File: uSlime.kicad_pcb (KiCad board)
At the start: 2 copper layers, 22.2 x 29.6 mm, 28 parts, among them J1 USB_C_4-LAYER_PADS, U1 ESP32-C6-WROOM-1-NARROW, U2 AP2112K-3.3TRG1, U3 MCP73831T-2ACI/OT, U5 BNO085, Y1 32.768

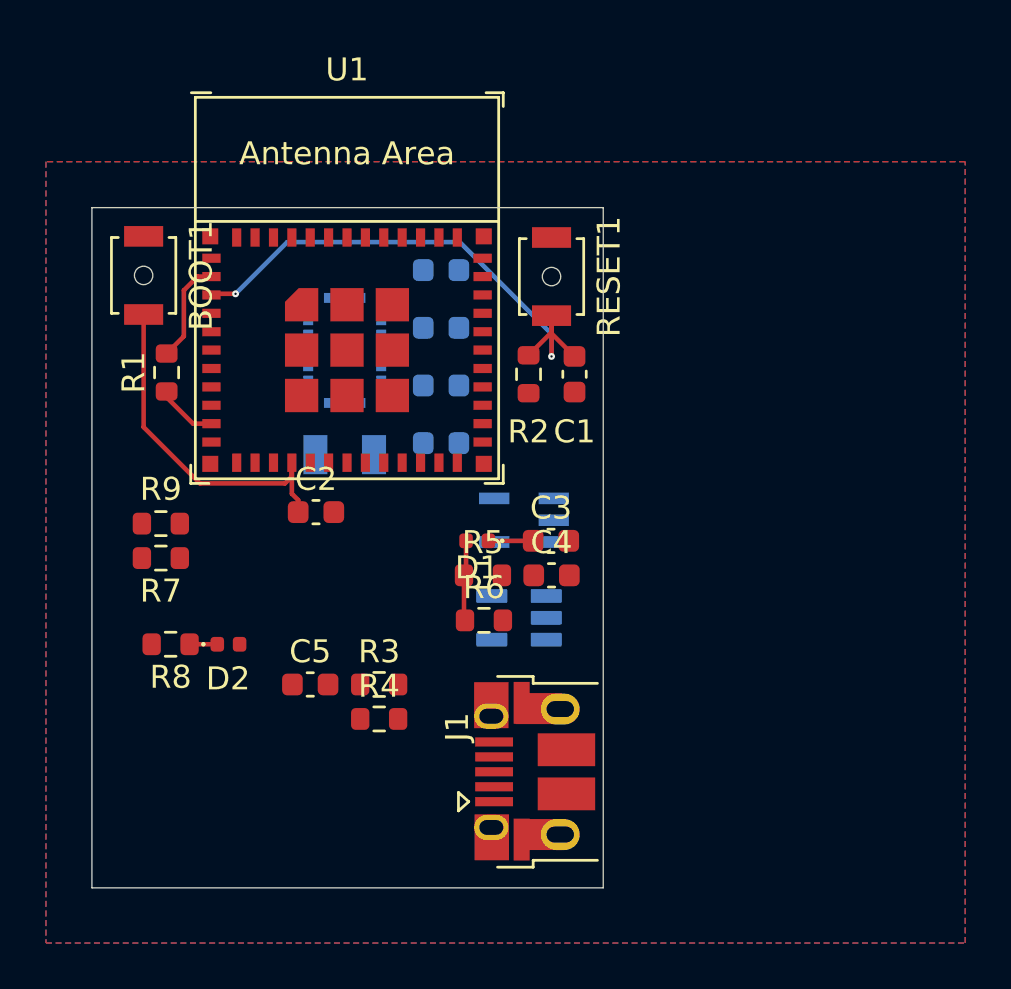
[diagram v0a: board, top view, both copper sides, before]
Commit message: update power
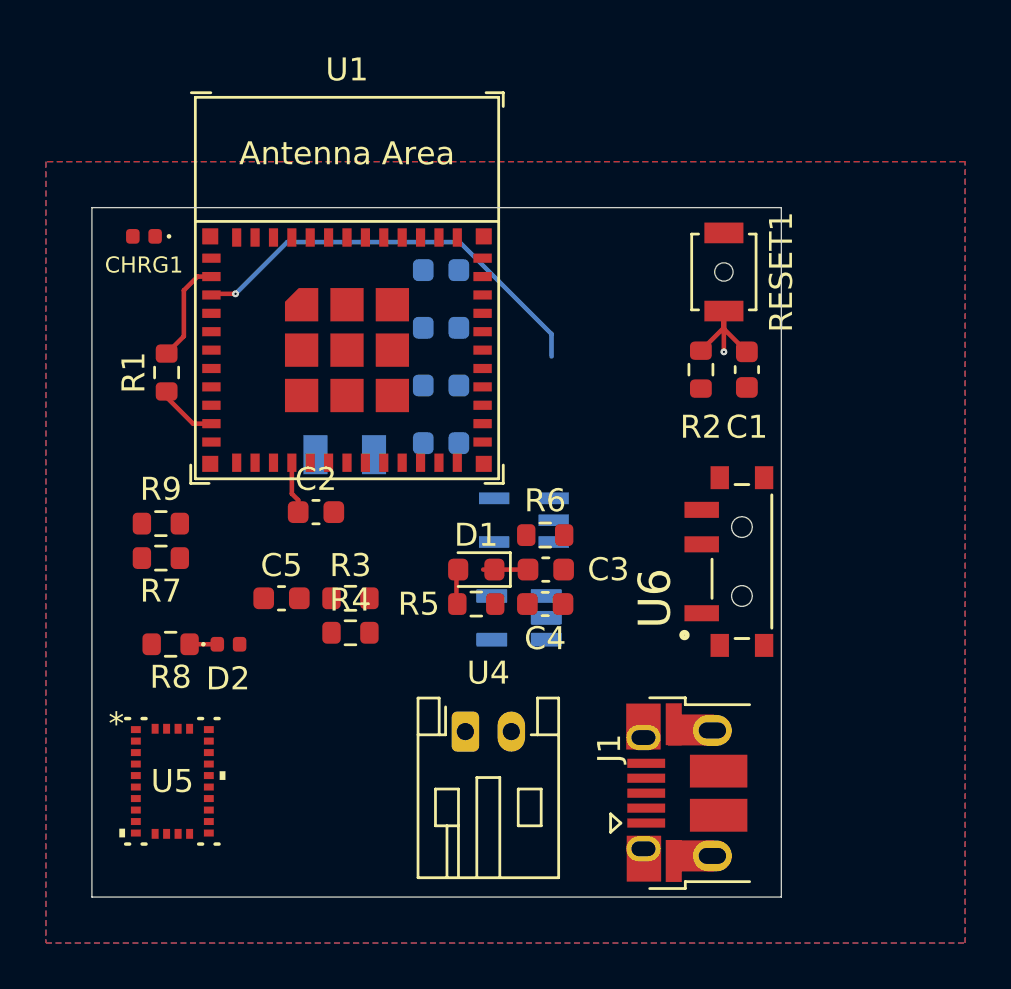
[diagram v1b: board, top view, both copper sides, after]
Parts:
- removed BOOT1: SW_Push, Button_Switch_SMD:SW_SPST_B3U-1000P-B
- added CHRG1: LED, LED_SMD:LED_0402_1005Metric, F.Cu at (102.9, 90.6)
- added U4: S2B-PH-K-S-GW, Connector_JST:JST_PH_S2B-PH-K_1x02_P2.00mm_Horizontal, F.Cu at (116.9, 112.2)
- added U6: MSK-12C02_SMD_SPDT_SWITCH, uSlime-libs:SW_PCM12SMTR, F.Cu at (128.9, 104.8)
- D1: footprint LED_SMD:LED_0402_1005Metric -> Diode_SMD:D_0603_1608Metric
- J1: value USB_C_4-LAYER_PADS -> USB_B_Micro
- R5: value 100k -> 390
- R6: value 390 -> 10K
- R7: value R -> 100K
- U5: moved to F.Cu
- moved U5 20.2 mm to (104.2, 114.3), turned to 0 degrees
- moved C1 7.50 mm to (129.2, 96.4)
- moved R2 7.50 mm to (127.2, 96.4)
- moved RESET1 7.50 mm to (128.2, 92.2)
- moved J1 6.69 mm to (126.5, 114.8)
- moved R6 4.57 mm to (120.4, 103.6)
- moved C5 3.95 mm to (108.9, 106.3)
- moved R3 3.95 mm to (111.9, 106.3)
- moved R4 3.95 mm to (111.9, 107.8)
- moved R5 1.28 mm to (117.4, 106.6)
- moved C4 1.28 mm to (120.4, 106.6)
- moved C3 1.27 mm to (120.4, 105.1)
- moved D1 1.25 mm to (117.4, 105.1)
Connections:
- C3 pad 1: Net-(D1-K) -> VBAT
- C4 pad 1: Net-(U2-VOUT) -> 3.3V
- C5 pad 1: unconnected-(C5-Pad1) -> GND
- C5 pad 2: unconnected-(C5-Pad2) -> VBAT
- C6 pad 1: unconnected-(C6-Pad1) -> GND
- D1 pad 1: Net-(D1-K) -> VBAT
- D1 pad 2: Net-(D1-A) -> VBUS
- J1 pad 1: V_USB -> VBUS
- J1 pad 2: /ESP32-C6FH4/USB_N -> D+ P
- J1 pad 3: /ESP32-C6FH4/USB_P -> D- N
- R5 pad 1: Net-(D1-A) -> VBUS
- R6 pad 1: Net-(D1-A) -> VBAT
- R6 pad 2: unconnected-(R6-Pad2) -> GND
- R7 pad 1: GND -> VBUS
- R7 pad 2: unconnected-(R7-Pad2) -> GND
- R8 pad 1: Net-(D2-K) -> Net-(CHRG1-K)
- R8 pad 2: unconnected-(R8-Pad2) -> Net-(U3-STAT)
- U1 pad 13: /ESP32-C6FH4/USB_N -> D- N
- U1 pad 14: /ESP32-C6FH4/USB_P -> D+ P
- U2 pad 1: Net-(D1-K) -> VBAT
- U2 pad 3: unconnected-(U2-EN-Pad3) -> VBAT
- U2 pad 5: Net-(U2-VOUT) -> 3.3V
- U3 pad 1: unconnected-(U3-STAT-Pad1) -> Net-(U3-STAT)
- U3 pad 2: unconnected-(U3-VSS-Pad2) -> GND
- U3 pad 3: unconnected-(U3-VBAT-Pad3) -> VBAT
- U3 pad 4: unconnected-(U3-VDD-Pad4) -> VBUS
- U3 pad 5: unconnected-(U3-PROG-Pad5) -> Net-(U3-PROG)
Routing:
- net /ESP32-C6FH4/IO9/BOOT: track 15.4 -> 2.26 mm
- net Net-(D1-A): track 3.52 -> 0.00 mm
- net VBAT: track 0.00 -> 1.95 mm
- net Net-(D1-K): track 1.95 -> 0.00 mm
- net VBUS: track 0.00 -> 1.52 mm
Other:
- board size 22.2 x 29.6 mm -> 30 x 30 mm
